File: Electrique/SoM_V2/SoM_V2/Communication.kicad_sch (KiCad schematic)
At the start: 27 parts, among them U301 TCA9546APWR, U302 MCP2515-xST, U303 TJA1051T, U304 FT231XS, Y301 8MHz

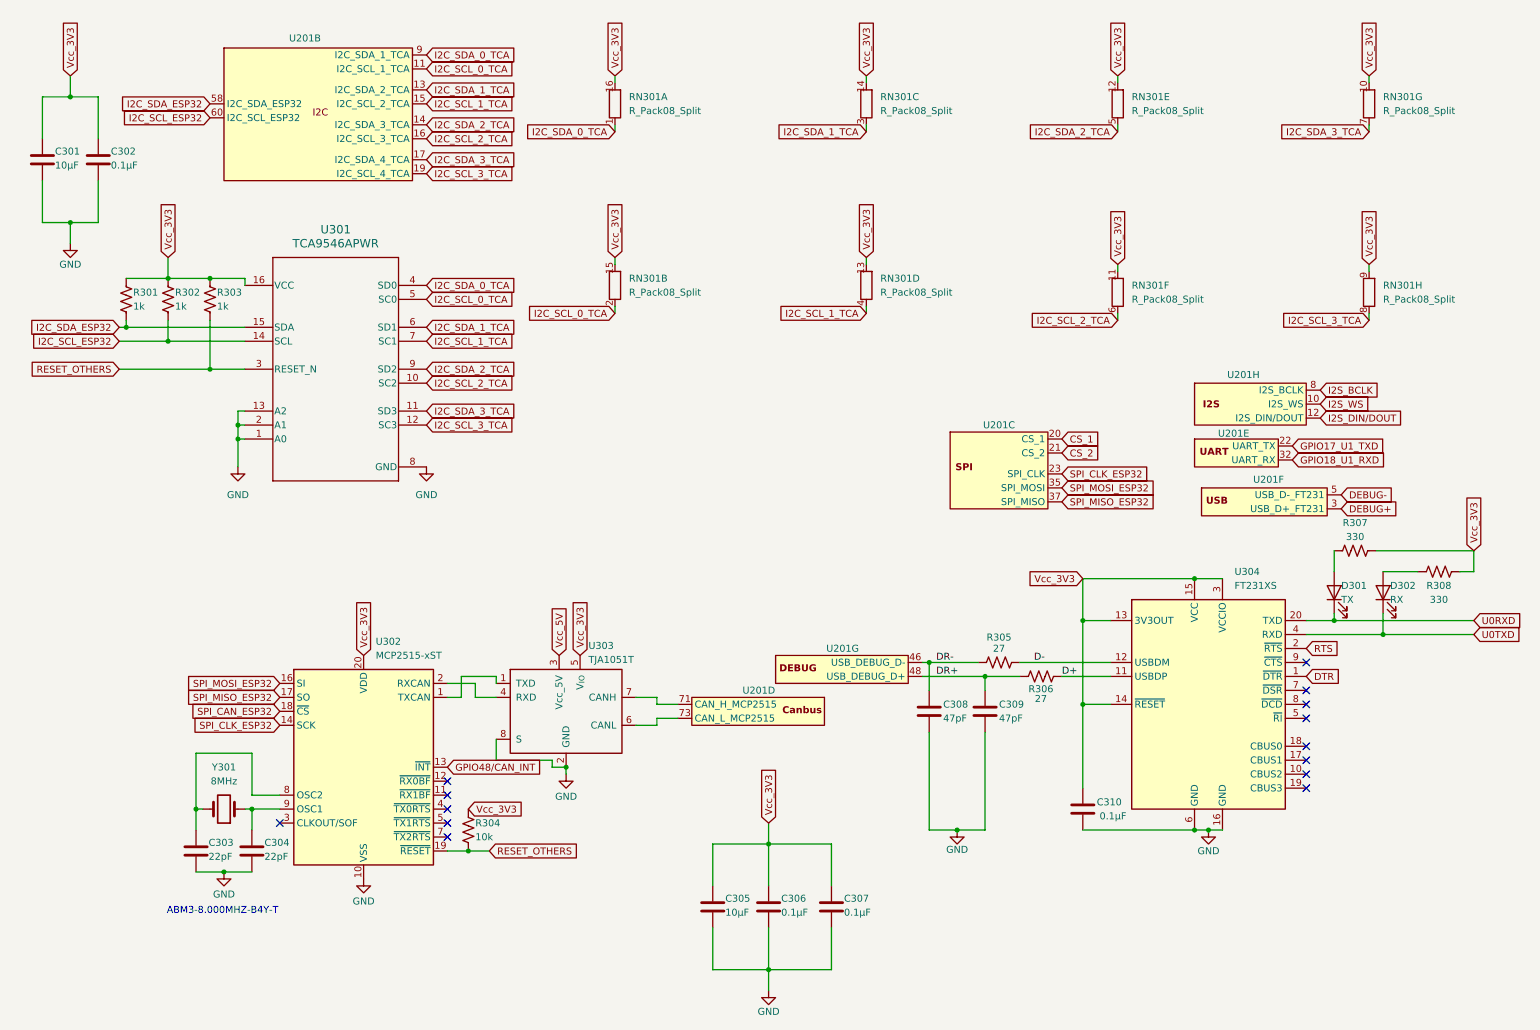
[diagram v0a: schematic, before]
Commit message: push v2.2
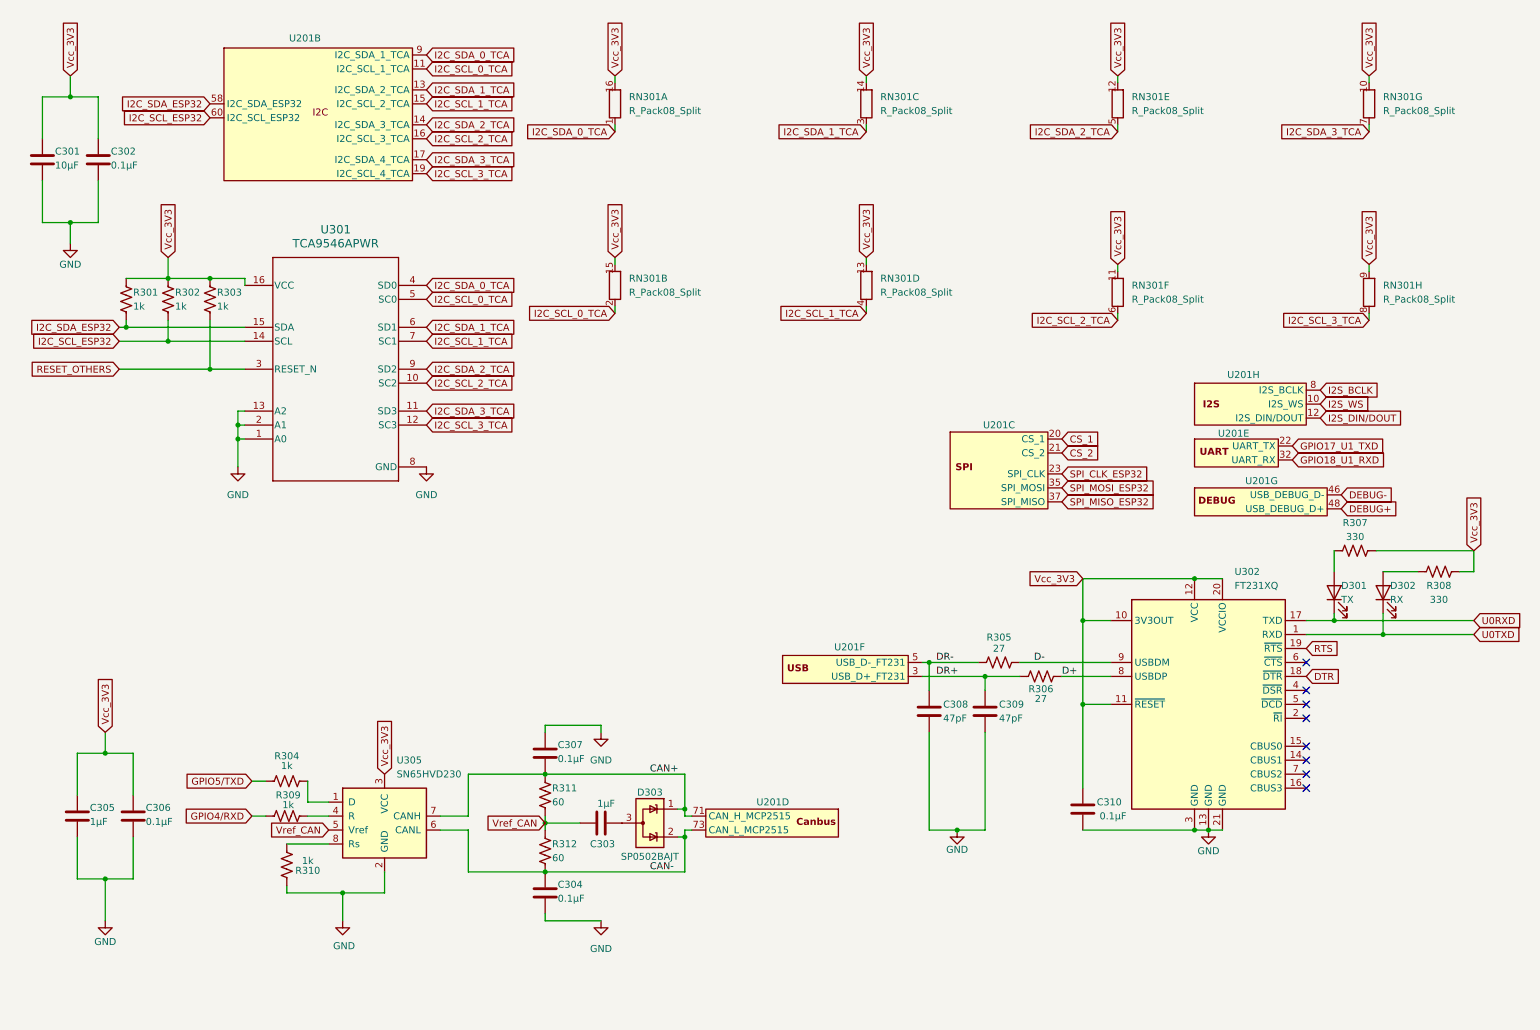
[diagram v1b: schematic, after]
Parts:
- removed U302: MCP2515-xST, Package_SO:TSSOP-20_4.4x6.5mm_P0.65mm, symbol Interface_CAN_LIN:MCP2515-xST
- removed U303: TJA1051T, Package_SO:SOIC-8_3.9x4.9mm_P1.27mm, symbol Interface_CAN_LIN:TJA1051T
- removed U304: FT231XS, Package_SO:SSOP-20_3.9x8.7mm_P0.635mm, symbol Interface_USB:FT231XS
- removed Y301: 8MHz, Crystal:Crystal_SMD_Abracon_ABM3-2Pin_5.0x3.2mm, symbol Device:Crystal
- added D303: SP0502BAJT, Package_TO_SOT_SMD:SOT-323_SC-70, symbol Power_Protection:SP0502BAJT
- added R309, R310: 1k, Resistor_SMD:R_0805_2012Metric, symbol Device:R_US
- added R311, R312: 60, Resistor_SMD:R_0805_2012Metric, symbol Device:R_US
- added U302: FT231XQ, Package_DFN_QFN:QFN-20-1EP_4x4mm_P0.5mm_EP2.5x2.5mm, symbol Interface_USB:FT231XQ
- added U305: SN65HVD230, Package_SO:SOIC-8_3.9x4.9mm_P1.27mm, symbol Interface_CAN_LIN:SN65HVD230
- C303: value 22pF -> 1µF
- C304: value 22pF -> 0.1µF
- C305: value 10µF -> 1µF
- R304: value 10k -> 1k
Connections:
- net D+: now also U302.8 (USBDP)
- net D-: now also U302.9 (USBDM)
- net DEBUG+: now also U201.48 (USB_DEBUG_D+); no longer U201.3 (USB_D+_FT231)
- net DEBUG-: now also U201.46 (USB_DEBUG_D-); no longer U201.5 (USB_D-_FT231)
- net DR+: now also U201.3 (USB_D+_FT231); no longer U201.48 (USB_DEBUG_D+)
- net DR-: now also U201.5 (USB_D-_FT231); no longer U201.46 (USB_DEBUG_D-)
- net DTR: now also U302.18 (~{DTR})
- net GND: now also C307.1, R310.1, U302.13 (GND), U302.21 (GND), U302.3 (GND), U305.2 (GND); no longer C303.2, C307.2
- net RESET_OTHERS: no longer R304.2
- net RTS: now also U302.19 (~{RTS})
- net U0RXD: now also U302.17 (TXD)
- net U0TXD: now also U302.1 (RXD)
- net Vcc_3V3: now also U302.10 (3V3OUT), U302.11 (~{RESET}), U302.12 (VCC), U302.20 (VCCIO), U305.3 (VCC); no longer C307.1, R304.1
- net CAN-: now reaches U201.73 (CAN_L_MCP2515)
- net CAN-: now also C304.1, D303.2 (K), R312.2, U305.6 (CANL)
- net CAN+: now reaches U201.71 (CAN_H_MCP2515)
- net CAN+: now also C307.2, D303.1 (K), R311.1, U305.7 (CANH)
- net Vref_CAN: now reaches C303.1
- net Vref_CAN: now also R311.2, R312.1, U305.5 (Vref)
- new net: R309.2, U305.4 (R)
- new net: C303.2, D303.3 (A)
- new net: R304.2, U305.1 (D)
- new net: R310.2, U305.8 (Rs)
- new net GPIO4/RXD: R309.1
- new net GPIO5/TXD: R304.1
- no-connect marks 14 -> 8
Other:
- note removed: "ABM3-8.000MHZ-B4Y-T"
- moved on the sheet: C305, C306, U201D, U201F, U201G
